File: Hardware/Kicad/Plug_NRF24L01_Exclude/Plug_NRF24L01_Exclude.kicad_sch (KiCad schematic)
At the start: 25 parts, among them J1 Conn_01x07_Socket, J2 Conn_01x08_Socket, Q1 2N7002, Q2 2N7002, Q3 2N7002, SW1 SW_Push, U2 AMS1117-3.3, U3 STM32L412KBTx

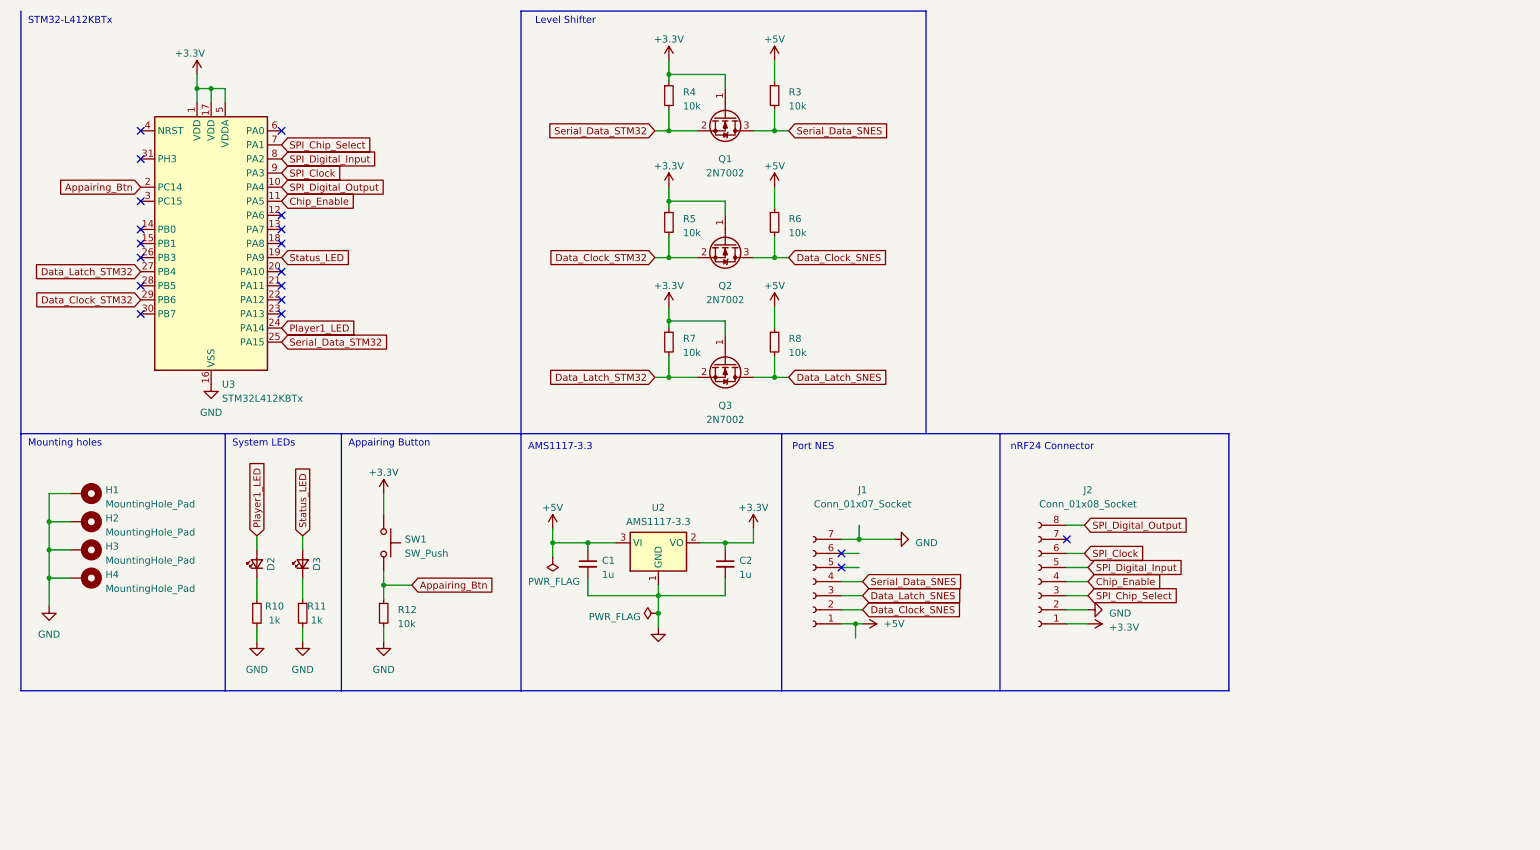
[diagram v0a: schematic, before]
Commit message: Corrective changes on the Plug_NRF24L01_Exclude KiCad
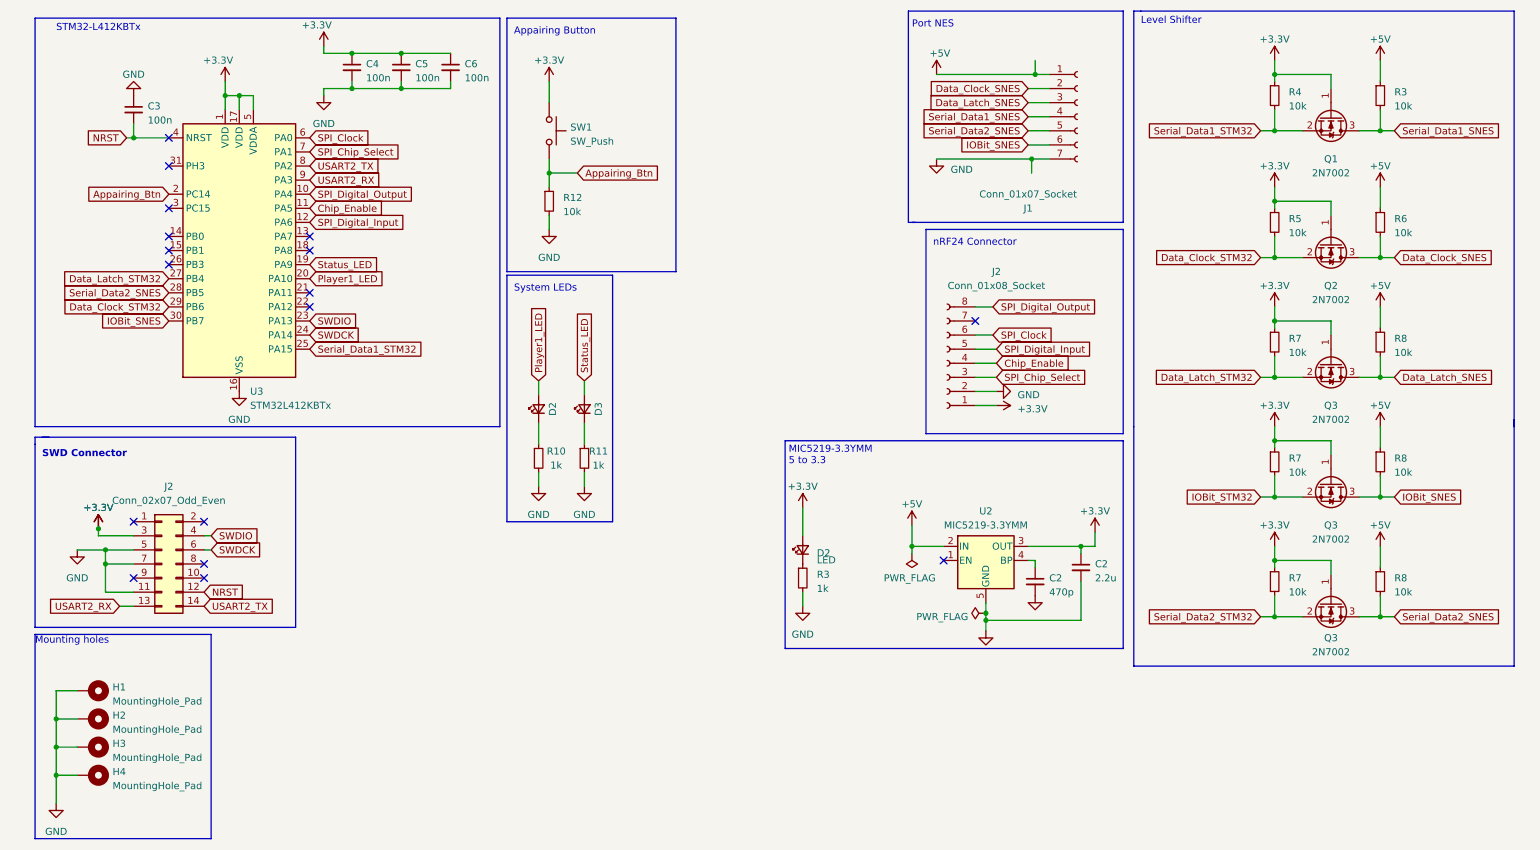
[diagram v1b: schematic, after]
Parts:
- removed C1: 1u, Capacitor_SMD:C_0603_1608Metric_Pad1.08x0.95mm_HandSolder, symbol Device:C_Small
- removed U2: AMS1117-3.3, Package_TO_SOT_SMD:SOT-223-3_TabPin2, symbol Regulator_Linear:AMS1117-3.3
- added C2: 470p, Capacitor_SMD:C_0603_1608Metric_Pad1.08x0.95mm_HandSolder, symbol Device:C_Small
- added C3, C4, C5, C6: 100n, Capacitor_SMD:C_0603_1608Metric_Pad1.08x0.95mm_HandSolder, symbol Device:C_Small
- added D2: LED, Diode_SMD:D_0603_1608Metric_Pad1.05x0.95mm_HandSolder, symbol Device:LED_Small
- added J2: Conn_02x07_Odd_Even, Connector_PinHeader_1.27mm:PinHeader_2x07_P1.27mm_Vertical_SMD, symbol Connector_Generic:Conn_02x07_Odd_Even
- added Q3 (x2): 2N7002, Package_TO_SOT_SMD:SOT-23, symbol Transistor_FET:2N7002
- added R3: 1k, Resistor_SMD:R_0603_1608Metric_Pad0.98x0.95mm_HandSolder, symbol Device:R_Small
- added R7 (x2), R8 (x2): 10k, Resistor_SMD:R_0603_1608Metric_Pad0.98x0.95mm_HandSolder, symbol Device:R_Small
- added U2: MIC5219-3.3YMM, Package_SO:MSOP-8_3x3mm_P0.65mm, symbol Regulator_Linear:MIC5219-3.3YMM
- C2: value 1u -> 2.2u
- J1: footprint Connector_PinSocket_1.00mm:PinSocket_1x07_P1.00mm_Vertical -> Connector_JST:JST_EH_B7B-EH-A_1x07_P2.50mm_Vertical
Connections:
- net +3.3V: now also C4.1, C5.1, C6.1, D2.2 (A), J2.3 (Pin_3), Q3.1 (G), Q3.1 (G), R7.1, R7.1, U2.3 (OUT)
- net +5V: now also R8.1, R8.1, U2.2 (IN)
- net GND: now also C2.2, C3.1, C4.2, C5.2, C6.2, J2.11 (Pin_11), J2.5 (Pin_5), J2.7 (Pin_7), R3.2, U2.5 (GND), U2.6 (GND), U2.7 (GND), U2.8 (GND)
- net Player1_LED: now also U3.20 (PA10); no longer U3.24 (PA14)
- net SPI_Clock: now also U3.6 (PA0); no longer U3.9 (PA3)
- net SPI_Digital_Input: now also U3.12 (PA6); no longer U3.8 (PA2)
- net SWDIO: now reaches U3.23 (PA13)
- net SWDIO: now also J2.4 (Pin_4)
- net Serial_Data2_SNES: now reaches U3.28 (PB5)
- net Serial_Data2_SNES: now also J1.5 (Pin_5), Q3.3 (D), R8.2
- net IOBit_SNES: now reaches U3.30 (PB7)
- net IOBit_SNES: now also J1.6 (Pin_6), Q3.3 (D), R8.2
- net NRST: now reaches U3.4 (NRST)
- net NRST: now also C3.2, J2.12 (Pin_12)
- net Serial_Data_SNES renamed Serial_Data1_SNES
- net Serial_Data_STM32 renamed Serial_Data1_STM32
- new net: C2.1, U2.4 (BP)
- new net: D2.1 (K), R3.1
- new net IOBit_STM32: Q3.2 (S), R7.2
- new net SWDCK: J2.6 (Pin_6), U3.24 (PA14)
- new net Serial_Data2_STM32: Q3.2 (S), R7.2
- new net USART2_RX: J2.13 (Pin_13), U3.9 (PA3)
- new net USART2_TX: J2.14 (Pin_14), U3.8 (PA2)
- no-connect marks 19 -> 17
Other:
- note added: "MIC5219-3.3YMM 5 to 3.3"
- note added: "SWD Connector"
- note removed: "AMS1117-3.3"
- moved on the sheet: C2, D2, D3, H1, H2, H3, H4, J1, J2, Q1, Q2, Q3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
